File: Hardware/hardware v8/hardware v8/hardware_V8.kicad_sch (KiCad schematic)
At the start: 36 parts, among them IC6 MLPF-WB-01E3, SW4 boot, U1 STM32WB55CGUx, Y1 830069528

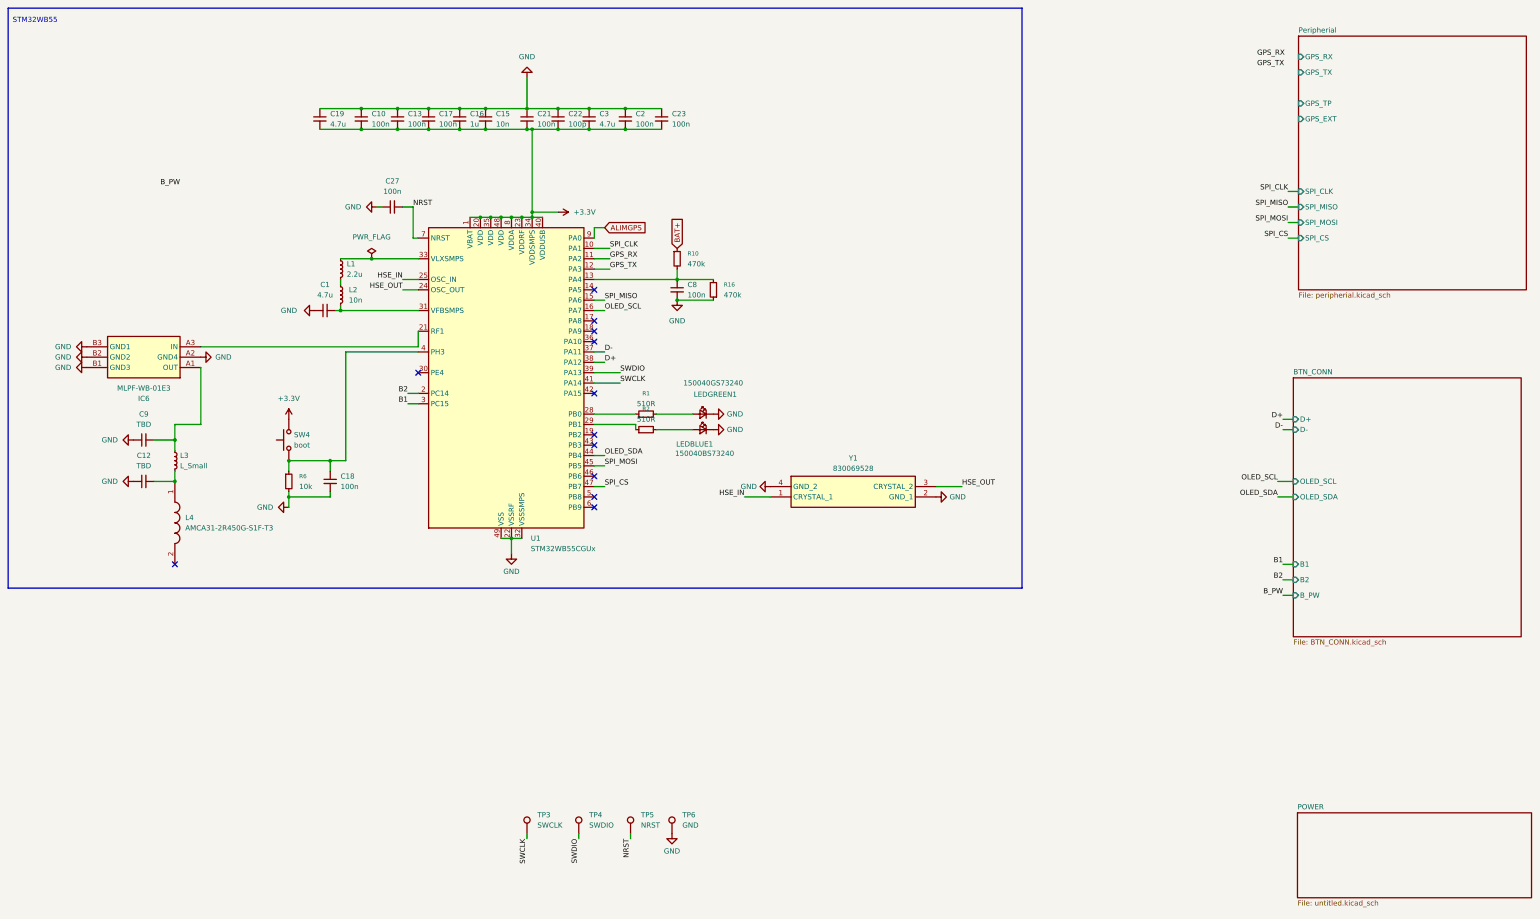
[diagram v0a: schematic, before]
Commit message: v8
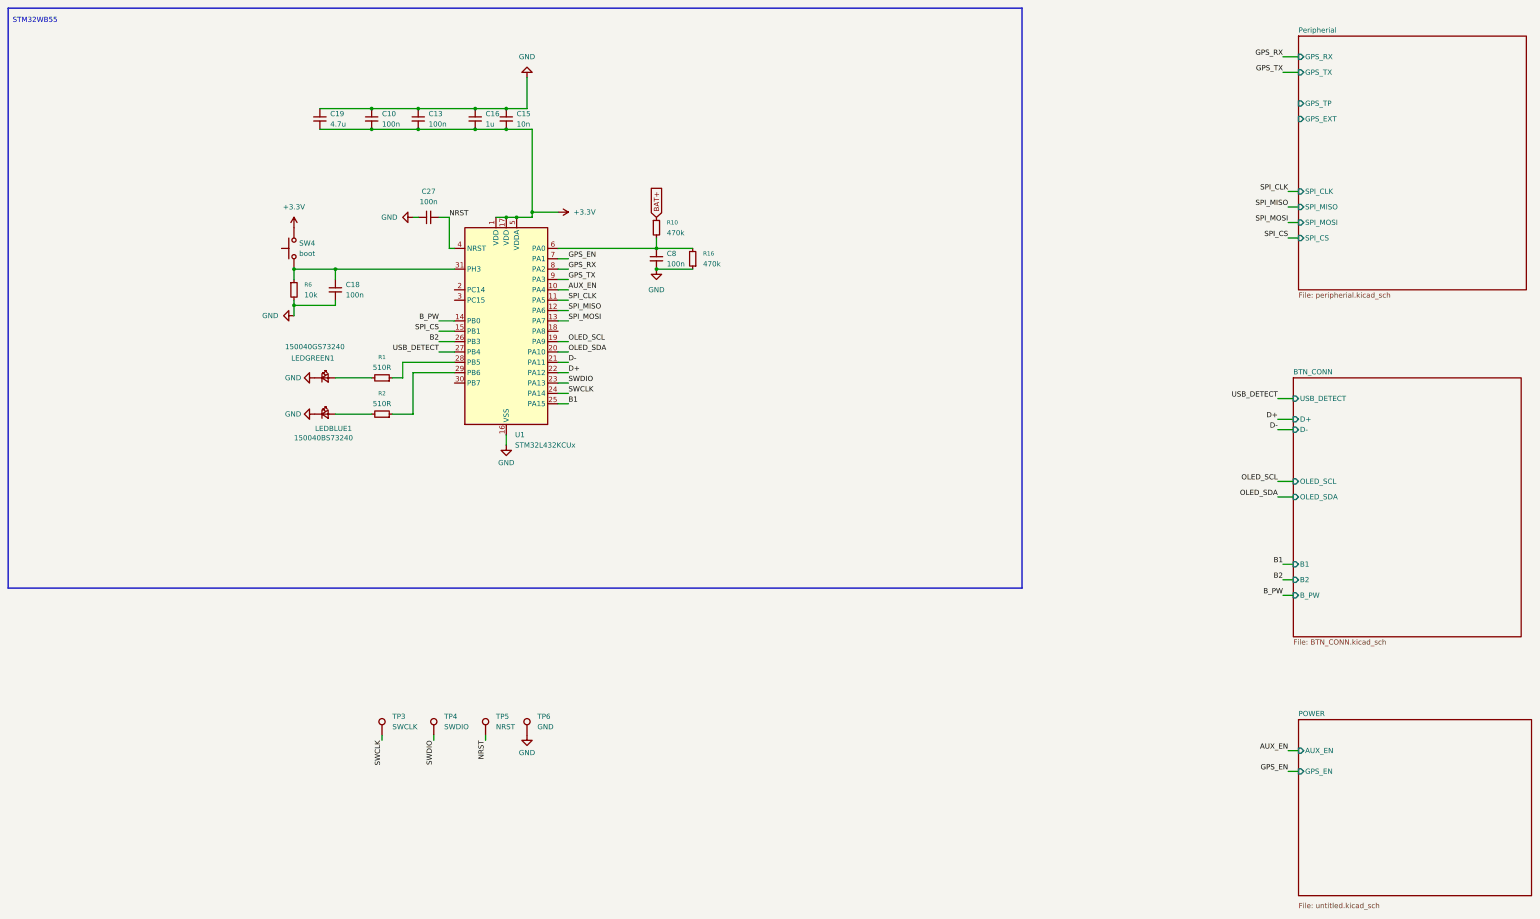
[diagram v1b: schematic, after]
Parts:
- removed C1, C3: 4.7u, Capacitor_SMD:C_0402_1005Metric, symbol Device:C_Small
- removed C12, C9: TBD, Capacitor_SMD:C_0201_0603Metric_Pad0.64x0.40mm_HandSolder, symbol Device:C_Small
- removed C17, C2, C21, C23: 100n, Capacitor_SMD:C_0201_0603Metric_Pad0.64x0.40mm_HandSolder, symbol Device:C_Small
- removed C22: 100p, Capacitor_SMD:C_0201_0603Metric_Pad0.64x0.40mm_HandSolder, symbol Device:C_Small
- removed IC6: MLPF-WB-01E3, samacsys2:BUMPLESS_CSP_2025, symbol samacsys2:MLPF-WB-01E3
- removed L1: 2.2u, Inductor_SMD:L_0805_2012Metric, symbol Device:L_Small
- removed L2: 10n, Inductor_SMD:L_0402_1005Metric, symbol Device:L_Small
- removed L3: L_Small, Inductor_SMD:L_0201_0603Metric_Pad0.64x0.40mm_HandSolder, symbol Device:L_Small
- removed L4: AMCA31-2R450G-S1F-T3, samacsys2:ANTC3216X140N, symbol samacsys2:AMCA31-2R450G-S1F-T3
- removed U1: STM32WB55CGUx, Package_DFN_QFN:QFN-48-1EP_7x7mm_P0.5mm_EP5.6x5.6mm, symbol MCU_ST_STM32WB:STM32WB55CGUx
- removed Y1: 830069528, samacsys:830069528, symbol samacsys:830069528
- added U1: STM32L432KCUx, Package_DFN_QFN:QFN-32-1EP_5x5mm_P0.5mm_EP3.45x3.45mm, symbol MCU_ST_STM32L4:STM32L432KCUx
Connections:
- net +3.3V: now also U1.1 (VDD), U1.17 (VDD), U1.5 (VDDA)
- net B1: now also U1.25 (PA15)
- net B2: now also U1.26 (PB3)
- net B_PW: now also U1.14 (PB0)
- net D+: now also U1.22 (PA12)
- net D-: now also U1.21 (PA11)
- net GND: now also U1.16 (VSS), U1.32 (VSS), U1.33 (VSS)
- net GPS_RX: now also U1.8 (PA2)
- net GPS_TX: now also U1.9 (PA3)
- net NRST: now also U1.4 (NRST)
- net OLED_SCL: now also U1.19 (PA9)
- net OLED_SDA: now also U1.20 (PA10)
- net SPI_CLK: now also U1.11 (PA5)
- net SPI_CS: now also U1.15 (PB1)
- net SPI_MISO: now also U1.12 (PA6)
- net SPI_MOSI: now also U1.13 (PA7)
- net SWCLK: now also U1.24 (PA14)
- net SWDIO: now also U1.23 (PA13)
- net at C8.1, R10.2, R16.2: now also U1.6 (PA0)
- net at R2.1: now also U1.29 (PB6)
- net at R1.1: now also U1.28 (PB5)
- net at C18.1, R6.1, SW4.1: now also U1.31 (PH3)
- new net AUX_EN: U1.10 (PA4)
- new net GPS_EN: U1.7 (PA1)
- new net USB_DETECT: U1.27 (PB4)
- no-connect marks 12 -> 0
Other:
- sheet BTN_CONN ports: added USB_DETECT; removed none
- sheet POWER ports: added AUX_EN, GPS_EN; removed none
- moved on the sheet: C10, C13, C15, C16, C18, C27, C8, LEDBLUE1, LEDGREEN1, R1, R10, R16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
